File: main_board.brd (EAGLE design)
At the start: 134.3 x 41.9 mm, 49 parts, among them IC1 LT1168ACS8, IC2 LT1168ACS8, IC3 LT1168ACS8, IC4 317EMP, U1 TLC272IP, U2 TLC272IP, U3 TLC272IP

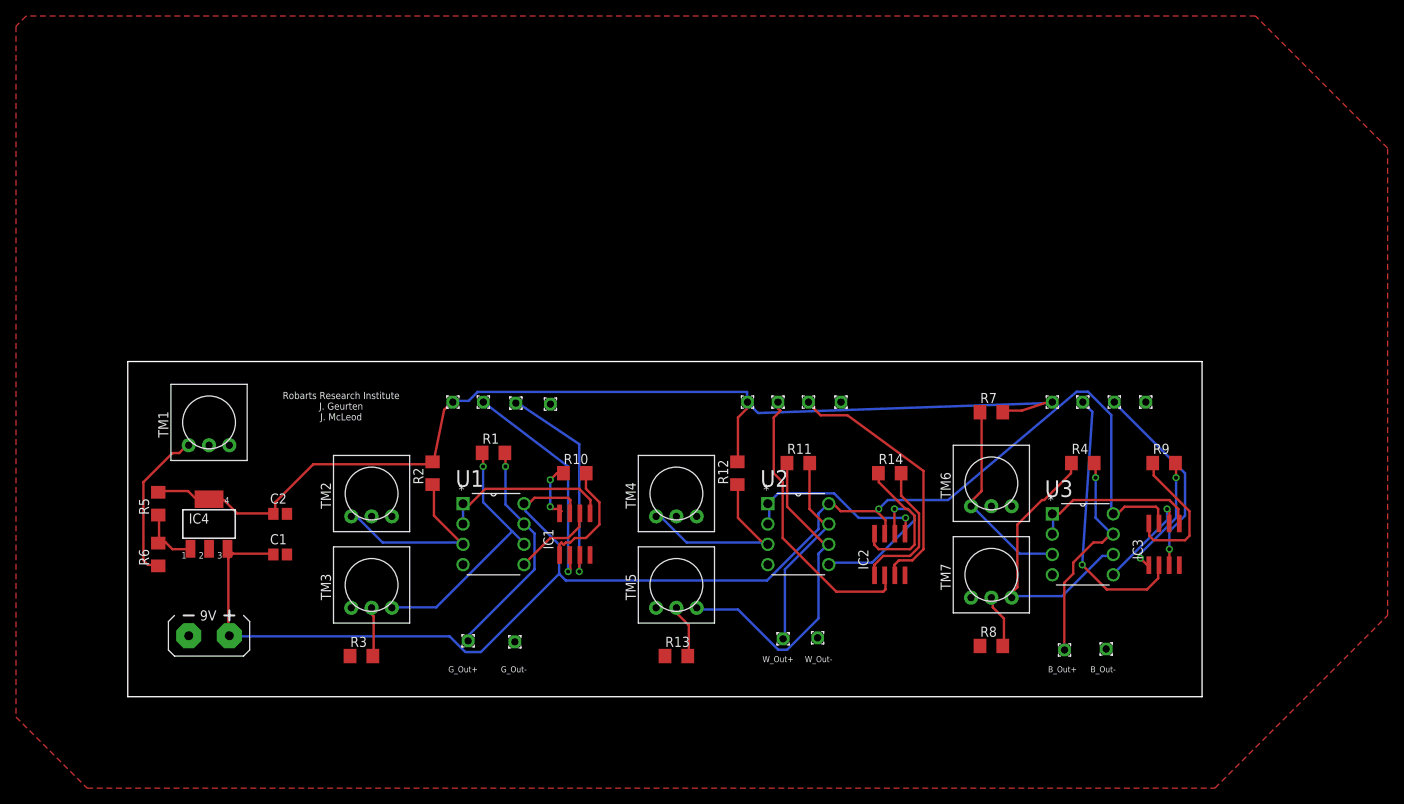
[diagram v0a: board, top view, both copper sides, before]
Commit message: Merging
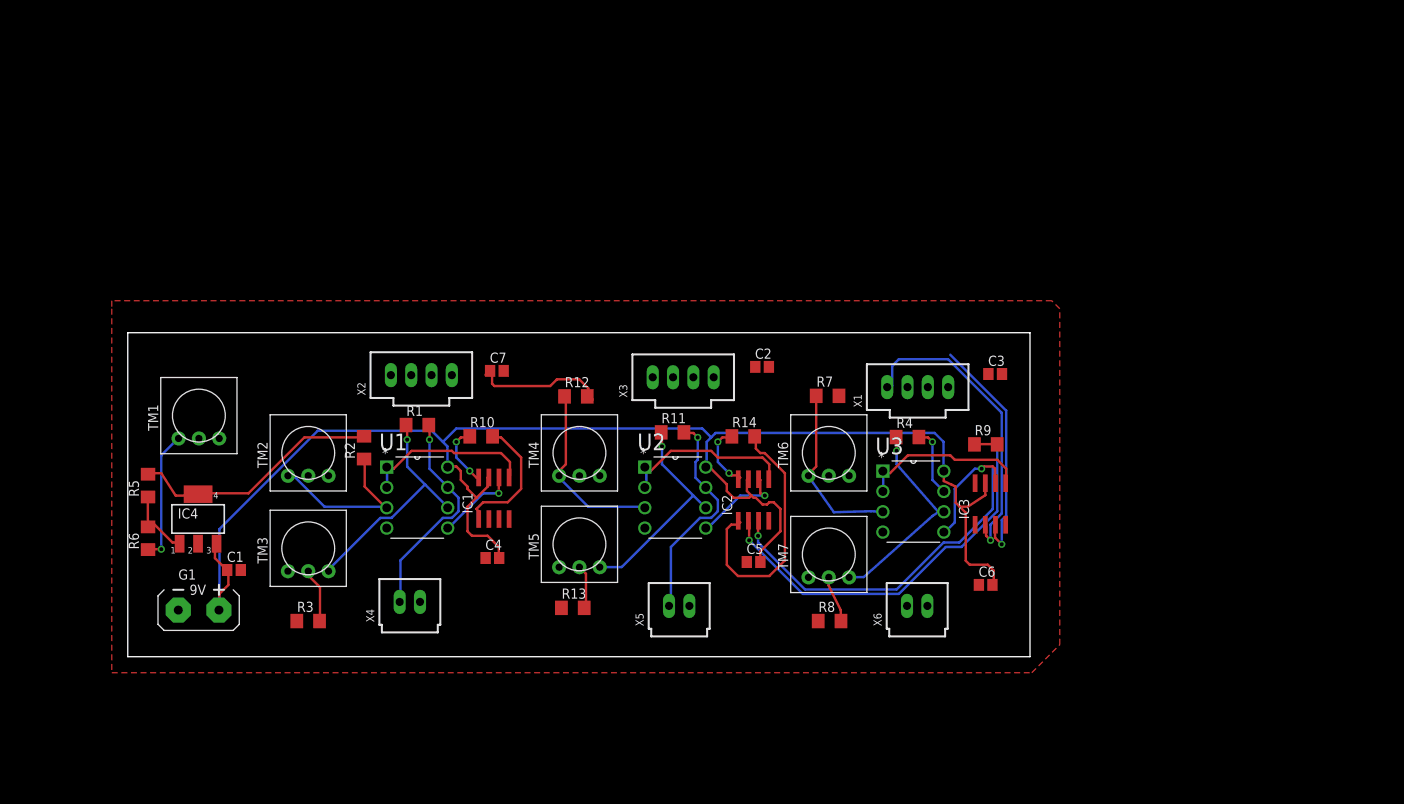
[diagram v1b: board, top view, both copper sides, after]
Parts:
- removed PAD1, PAD10, PAD11, PAD12, PAD2, PAD25, PAD26, PAD27, PAD28, PAD29, PAD3, PAD30, PAD4, PAD5, PAD6, PAD7, PAD8, PAD9: (no value), wirepad:1,6/0,9
- added C3, C4, C5, C6, C7: 10uF, adafruit:C2012
- added X1, X2, X3: C-GRID-04-70543, con-molex:70543-04
- added X4, X5, X6: C-GRID-02-70543, con-molex:70543-02
- C1: value (none) -> 1uF; device eagle-ltspice:C2012 -> adafruit:C2012
- C2: value (none) -> 10uF; device eagle-ltspice:C2012 -> adafruit:C2012
- R13, R7: value (none) -> 30kO
- moved C2 63.0 mm to (79.3, 41.2)
- moved R9 22.4 mm to (107.3, 31.5)
- moved R12 22.3 mm to (56.0, 37.5), turned to 0 degrees
- moved IC3 22.3 mm to (107.8, 24.1)
- moved R4 22.1 mm to (97.5, 32.5)
- moved U3 21.8 mm to (102.0, 20.6)
- moved TM6 20.7 mm to (87.6, 30.5)
- moved R7 20.6 mm to (87.5, 37.6)
- moved TM7 20.5 mm to (87.6, 17.8)
- moved R8 20.5 mm to (87.7, 9.46)
- moved R14 18.9 mm to (76.9, 32.5)
- moved IC2 18.3 mm to (78.2, 24.6)
- moved R11 16.2 mm to (68.1, 33.0)
- moved U2 16.0 mm to (72.2, 21.1)
- moved R13 14.3 mm to (55.6, 11.1)
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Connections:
- net N$11 renamed U3_1_IN+
- net N$12 renamed IC3_RG1
- net N$13 renamed TM7POT2
- net N$14 renamed IC3_RG8
- net N$15 renamed U3_2_IN+
- net N$2 renamed U1_2IN-
- net N$20 renamed U1_2IN+
- net N$24 renamed U2_2IN-
- net N$25 renamed U2_1IN+
- net N$26 renamed U2_1IN-
- net N$27 renamed TM5POT2
- net N$3 renamed U1_1IN+
- net N$30 renamed U2_2IN+
- net N$4 renamed U1_1IN-
- net N$5 renamed TM2POT2
- net N$6 renamed ADJ
- net N$8 renamed U3_2_IN-
- net N$9 renamed U3_1_IN-
- removed net N$17: IC3.3, PAD2.1
- removed net N$18: IC3.2, PAD1.1
- removed net N$21: IC1.3, PAD26.1
- removed net N$22: IC1.2, PAD25.1
- removed net N$31: IC2.3, PAD29.1
- removed net N$32: IC2.2, PAD28.1
- new net BLUE_IN_B: IC3.3, X1.2
- new net BLUE_IN_R: IC3.2, X1.3
- new net GREEN_IN_B: IC1.3, X2.2
- new net GREEN_IN_R: IC1.2, X2.3
- new net WHITE_IN_B: IC2.3, X3.2
- new net WHITE_IN_R: IC2.2, X3.3
- net GND: now also C3.2, C4.1, C5.1, C6.1, C7.2, X1.4, X2.4, X3.4, X4.2, X5.2, X6.2; no longer PAD10.1, PAD11.1, PAD12.1, PAD7.1, PAD8.1, PAD9.1
- net N$1: now also X4.1; no longer PAD27.1
- net N$23: now also X5.1; no longer PAD30.1
- net N$7: no longer PAD3.1
- net VCC: now also C4.2, C5.2, C6.2
- net VDD: now also C3.1, C7.1, X1.1, X2.1, X3.1; no longer PAD4.1, PAD5.1, PAD6.1
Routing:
- net VDD: track 139.6 -> 49.7 mm
- net WHITE_IN_R: track 0.00 -> 48.1 mm, vias 0 -> 1
- net WHITE_IN_B: track 0.00 -> 44.0 mm, vias 0 -> 1
- net BLUE_IN_R: track 0.00 -> 39.6 mm, vias 0 -> 1
- net N$32: track 35.5 -> 0.00 mm
- net N$18: track 33.9 -> 0.00 mm, vias 1 -> 0
- net N$31: track 33.2 -> 0.00 mm
- net BLUE_IN_B: track 0.00 -> 29.6 mm, vias 0 -> 1
- net N$22: track 28.6 -> 0.00 mm, vias 1 -> 0
- net N$21: track 27.5 -> 0.00 mm, vias 1 -> 0
- net N$17: track 24.9 -> 0.00 mm, vias 1 -> 0
- net N$7: track 27.9 -> 8.74 mm
- net IC3_RG8: track 18.0 -> 2.58 mm
- net IC3_RG1: track 15.2 -> 0.00 mm, vias 2 -> 0
- net N$28: track 18.0 -> 32.9 mm
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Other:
- board size 134.3 x 41.9 mm -> 112.8 x 40.5 mm
- board text removed: "B_Out+"
- board text removed: "B_Out-"
- board text removed: "G_Out+"
- board text removed: "G_Out-"
- board text removed: "Robarts Research Institute J. Geurten J. McLeod"
- board text removed: "W_Out+"
- board text removed: "W_Out-"
